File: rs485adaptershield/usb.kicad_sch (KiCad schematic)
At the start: 15 parts, among them IC1 USB2422-I_MJ, U8 AP2171W

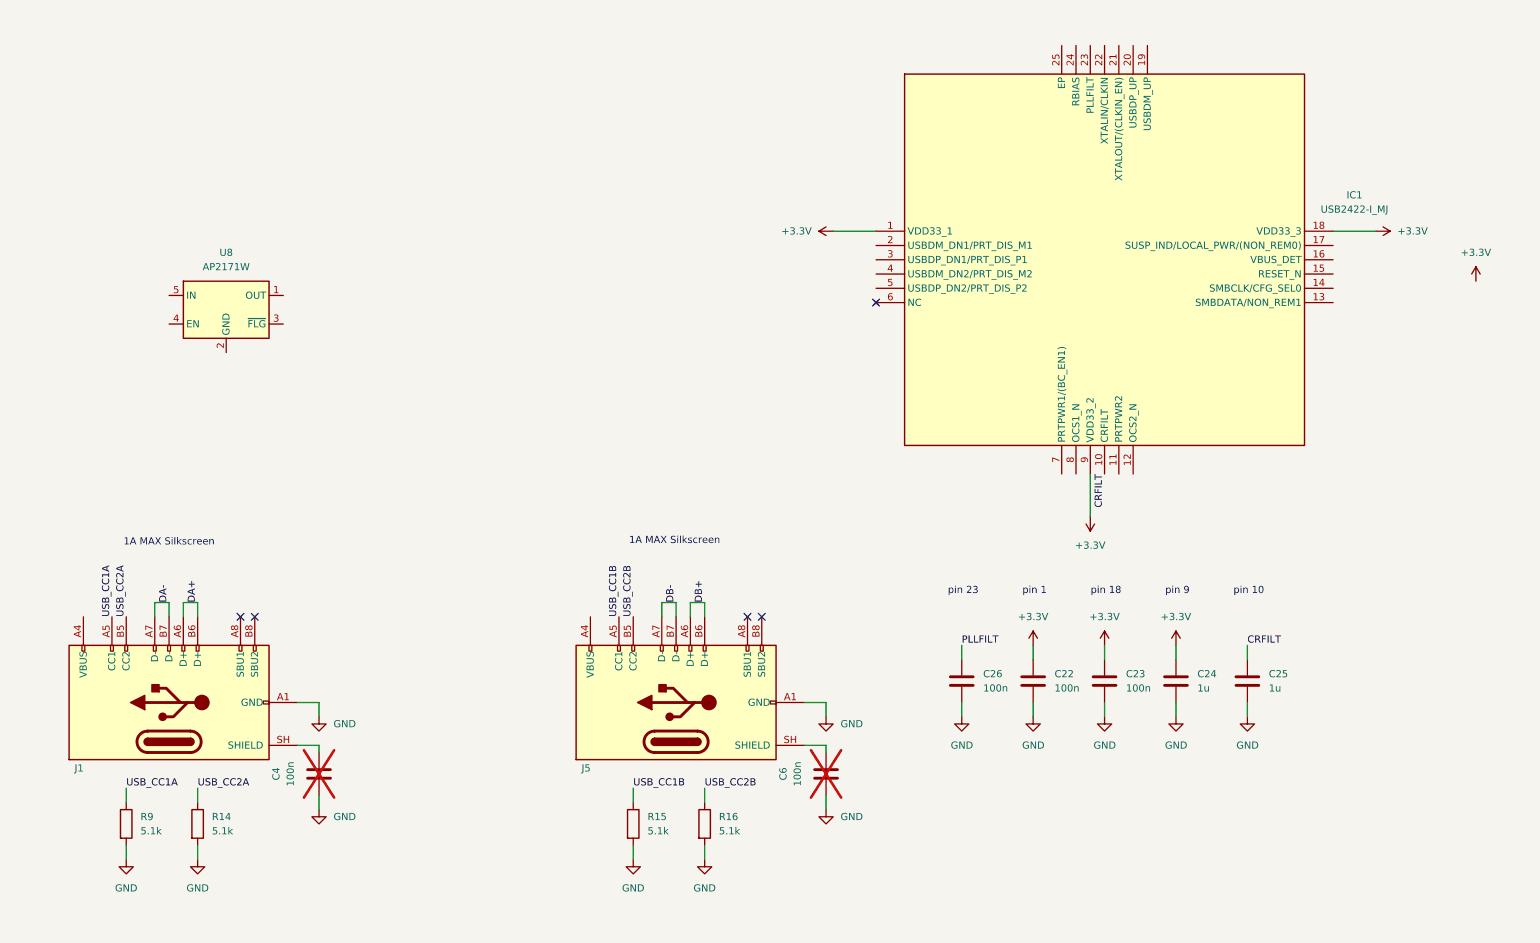
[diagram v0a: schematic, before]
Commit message: more progress
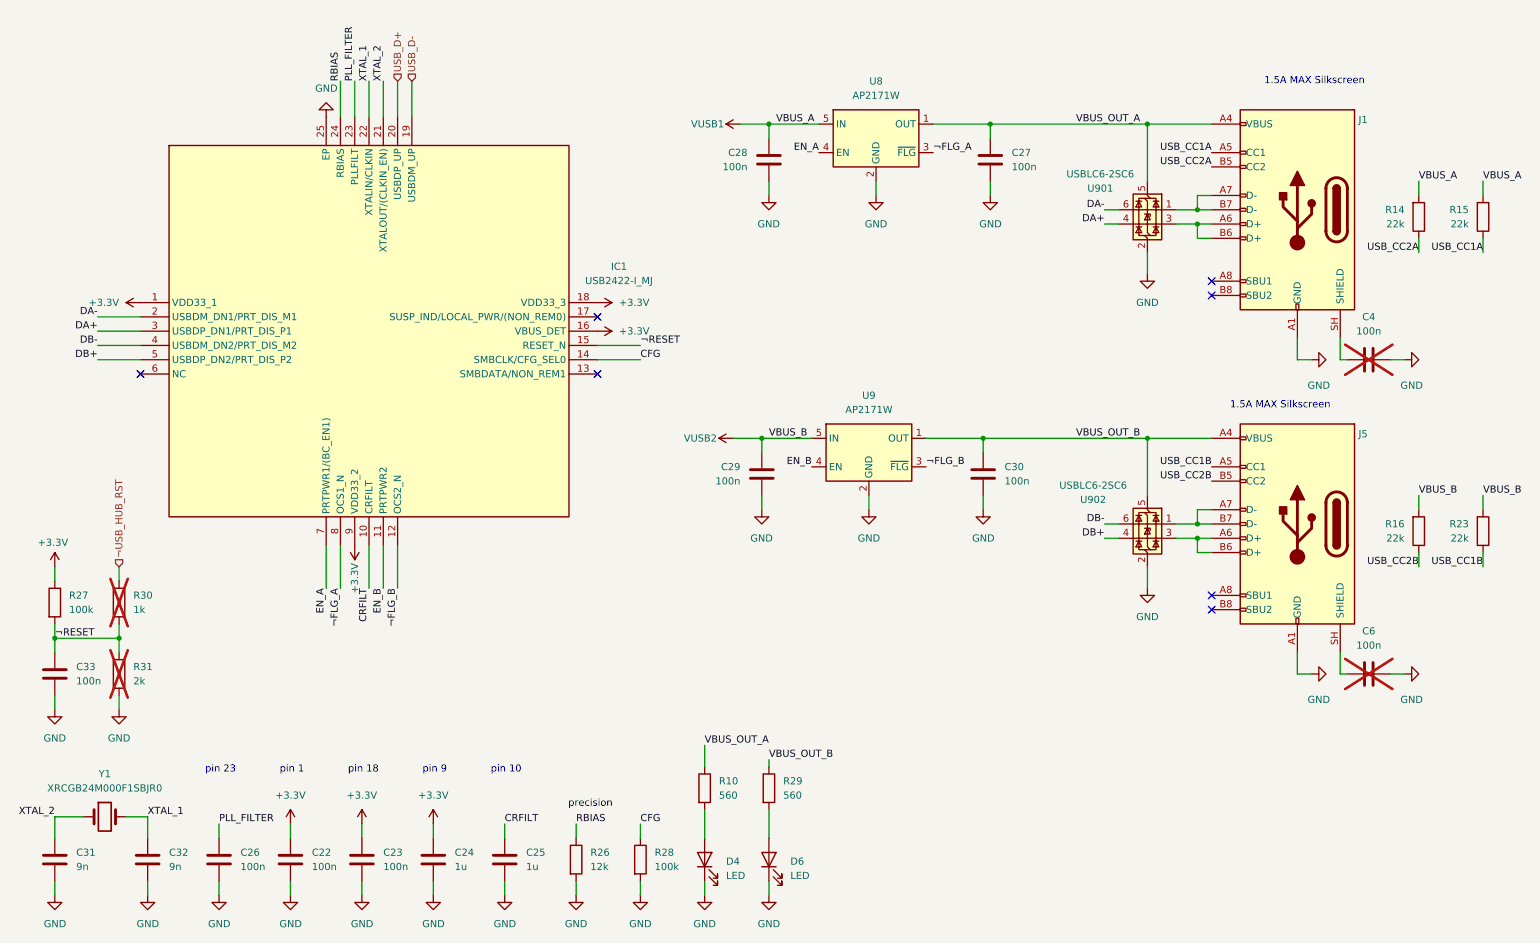
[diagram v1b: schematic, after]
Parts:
- removed R9: 5.1k, Capacitor_SMD:C_0402_1005Metric, symbol Device:R
- added C27, C28, C29, C30, C33: 100n, Capacitor_SMD:C_0603_1608Metric, symbol Device:C
- added C31, C32: 9n, Capacitor_SMD:C_0603_1608Metric, symbol Device:C
- added D4, D6: LED, LED_SMD:LED_0805_2012Metric, symbol Device:LED
- added R10, R29: 560, Resistor_SMD:R_0805_2012Metric, symbol Device:R
- added R23: 22k, Capacitor_SMD:C_0402_1005Metric, symbol Device:R
- added R26: 12k, Capacitor_SMD:C_0402_1005Metric, symbol Device:R
- added R27, R28: 100k, Capacitor_SMD:C_0402_1005Metric, symbol Device:R
- added R30: 1k, Capacitor_SMD:C_0402_1005Metric, symbol Device:R
- added R31: 2k, Capacitor_SMD:C_0402_1005Metric, symbol Device:R
- added U9: AP2171W, Package_TO_SOT_SMD:SOT-23-5, symbol Power_Management:AP2171W
- added U901, U902: USBLC6-2SC6, Package_TO_SOT_SMD:SOT-23-6, symbol Power_Protection:USBLC6-2SC6
- added Y1: XRCGB24M000F1SBJR0, symbol Device:Crystal
- R14, R15, R16: value 5.1k -> 22k
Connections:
- net PLLFILT is gone; now on net PLL_FILTER: C26.2
- net +3.3V: now also IC1.16 (VBUS_DET), R27.1
- net DA+: now also IC1.3 (USBDP_DN1/PRT_DIS_P1), U901.4 (I/O2); no longer J1.A6 (D+), J1.B6 (D+)
- net DA-: now also IC1.2 (USBDM_DN1/PRT_DIS_M1), U901.6 (I/O1); no longer J1.A7 (D-), J1.B7 (D-)
- net DB+: now also IC1.5 (USBDP_DN2/PRT_DIS_P2), U902.4 (I/O2); no longer J5.A6 (D+), J5.B6 (D+)
- net DB-: now also IC1.4 (USBDM_DN2/PRT_DIS_M2), U902.6 (I/O1); no longer J5.A7 (D-), J5.B7 (D-)
- net GND: now also IC1.25 (EP), U8.2 (GND), C27.1, C28.1, C29.1, C30.1, C31.1, C32.1, C33.1, D4.1 (K), D6.1 (K), R26.2, R28.2, R31.2, U9.2 (GND), U901.2 (GND), U902.2 (GND); no longer R14.2, R15.2, R16.2
- net USB_CC1A: now also R15.1
- net USB_CC1B: now also R23.1; no longer R15.1
- net VBUS_OUT_A: now reaches U8.1 (OUT)
- net VBUS_OUT_A: now also J1.A4 (VBUS), J1.A9 (VBUS), J1.B4 (VBUS), J1.B9 (VBUS), C27.2, R10.1, U901.5 (VBUS)
- net ¬FLG_A: now reaches U8.3 (~{FLG})
- net ¬FLG_A: now also IC1.8 (OCS1_N)
- net EN_A: now reaches U8.4 (EN)
- net EN_A: now also IC1.7 (PRTPWR1/(BC_EN1))
- net VUSB1: now reaches U8.5 (IN)
- net VUSB1: now also R14.2, R15.2, C28.2
- net VBUS_OUT_B: now reaches J5.A4 (VBUS), J5.A9 (VBUS), J5.B4 (VBUS), J5.B9 (VBUS)
- net VBUS_OUT_B: now also C30.2, R29.1, U9.1 (OUT), U902.5 (VBUS)
- net EN_B: now reaches IC1.11 (PRTPWR2)
- net EN_B: now also U9.4 (EN)
- net ¬FLG_B: now reaches IC1.12 (OCS2_N)
- net ¬FLG_B: now also U9.3 (~{FLG})
- net CFG: now reaches IC1.14 (SMBCLK/CFG_SEL0)
- net CFG: now also R28.1
- net ¬RESET: now reaches IC1.15 (RESET_N)
- net ¬RESET: now also C33.2, R27.2, R30.2, R31.1
- net USB_D-: now reaches IC1.19 (USBDM_UP)
- net USB_D+: now reaches IC1.20 (USBDP_UP)
- net XTAL_2: now reaches IC1.21 (XTALOUT/(CLKIN_EN))
- net XTAL_2: now also C31.2, Y1.1
- net XTAL_1: now reaches IC1.22 (XTALIN/CLKIN)
- net XTAL_1: now also C32.2, Y1.2
- net PLL_FILTER: now reaches IC1.23 (PLLFILT)
- net RBIAS: now reaches IC1.24 (RBIAS)
- net RBIAS: now also R26.1
- new net: J1.A7 (D-), J1.B7 (D-), U901.1 (I/O1)
- new net: J1.A6 (D+), J1.B6 (D+), U901.3 (I/O2)
- new net: J5.A7 (D-), J5.B7 (D-), U902.1 (I/O1)
- new net: J5.A6 (D+), J5.B6 (D+), U902.3 (I/O2)
- new net: D4.2 (A), R10.2
- new net: D6.2 (A), R29.2
- new net VUSB2: C29.2, R16.2, R23.2, U9.5 (IN)
- new net ¬USB_HUB_RST: R30.1
- no-connect marks 5 -> 7
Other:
- note added: "1.5A MAX Silkscreen"
- note added: "precision"
- note removed: "1A MAX Silkscreen"
- moved on the sheet: C22, C23, C24, C25, C26, C4, C6, IC1, J1, J5, R14, U8
